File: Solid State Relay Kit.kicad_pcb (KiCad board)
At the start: 2 copper layers, 25.8 x 21 mm, 11 parts, among them J1 Conn_01x03, J2 Conn_01x02, Q1 2N3904, U1 S108T02

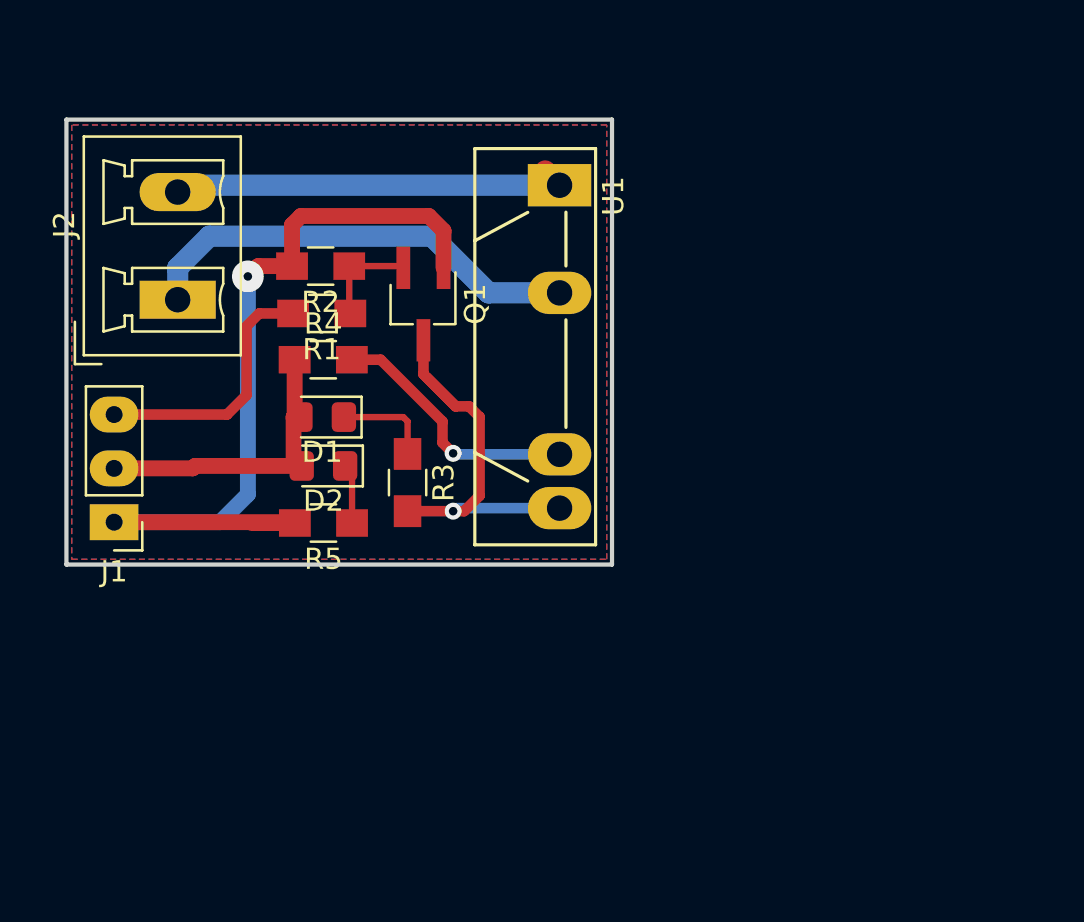
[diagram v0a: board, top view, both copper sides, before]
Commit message: update,
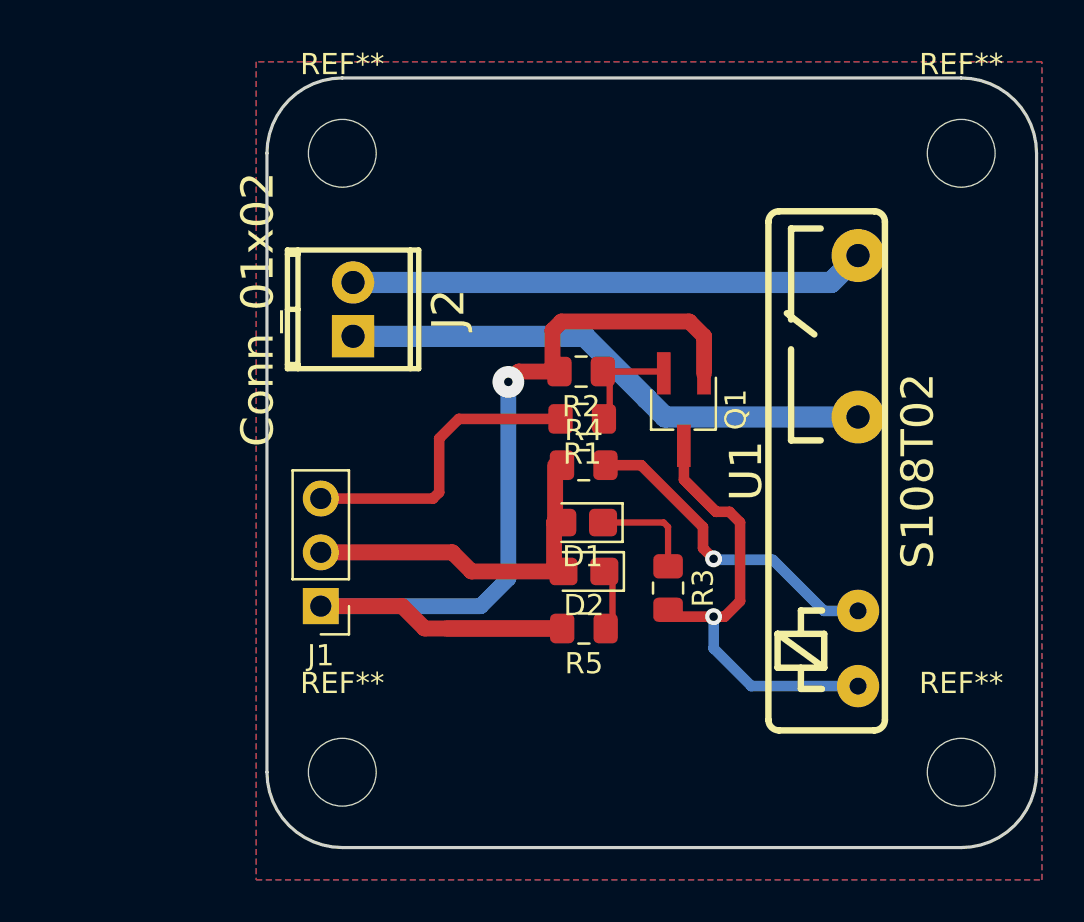
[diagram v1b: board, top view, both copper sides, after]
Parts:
- added REF**: MountingHole_3.2mm_M3, MountingHole:MountingHole_3.2mm_M3, F.Cu at (33.0, 21.6)
- added REF**: MountingHole_3.2mm_M3, MountingHole:MountingHole_3.2mm_M3, F.Cu at (33.0, 50.8)
- added REF**: MountingHole_3.2mm_M3, MountingHole:MountingHole_3.2mm_M3, F.Cu at (62.2, 21.6)
- added REF**: MountingHole_3.2mm_M3, MountingHole:MountingHole_3.2mm_M3, F.Cu at (62.2, 50.8)
- D1, D2: footprint LED_SMD:LED_0805_2012Metric_Pad1.15x1.40mm_HandSolder -> LED_SMD:LED_0805_2012Metric_Castellated
- J1: footprint footprint-lib.pretty:Pin_Header_Straight_1x03_Pitch2.54mm -> Connector_PinHeader_2.54mm:PinHeader_1x03_P2.54mm_Vertical
- J2: footprint Connectors_Phoenix:PhoenixContact_MCV-G_02x5.08mm_Vertical -> w_conn_mpt:mpt_0,5%2f2-2,54
- R1, R2, R3, R4, R5: footprint footprint-lib.pretty:R_0805_HandSoldering -> Resistor_SMD:R_0805_2012Metric_Pad1.15x1.40mm_HandSolder
- U1: footprint Housings_SIP:SIP4_Sharp-SSR_Pitch7.62mm_Straight -> footprint-lib:OMRON-G3MB-202P
- moved U1 18.5 mm to (55.9, 36.6), turned to 90 degrees
- moved D2 13.3 mm to (44.4, 41.3)
- moved R3 13.3 mm to (48.4, 42.1)
- moved R4 13.3 mm to (44.4, 36.3)
- moved R5 13.3 mm to (44.4, 44.0)
- moved R1 13.3 mm to (44.3, 34.1)
- moved R2 13.3 mm to (44.3, 31.9)
- moved D1 13.3 mm to (44.4, 39.0)
- moved Q1 13.3 mm to (49.1, 33.7)
- moved J1 10.5 mm to (32.0, 43.0)
- moved J2 8.29 mm to (33.5, 29.0), turned to 270 degrees
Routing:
- net GND: track 41.3 -> 49.6 mm
- net /SSR_OUT2: track 19.1 -> 24.4 mm
- net /SSR_IN1: track 19.7 -> 23.7 mm
- net /SSR_OUT1: track 22.1 -> 25.4 mm
- net +5V: track 13.6 -> 16.5 mm
- net /SSR_IN2: track 13.6 -> 16.4 mm
- net /SIG_CONTROL: track 12.3 -> 14.4 mm
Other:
- board size 25.8 x 21 mm -> 36.3 x 36.3 mm
